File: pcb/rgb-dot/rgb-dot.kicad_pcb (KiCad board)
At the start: 2 copper layers, 7.6 x 8.9 mm, 4 parts, among them J1 HEADER-1x03, J2 HEADER-1x03, U1 WS2812B

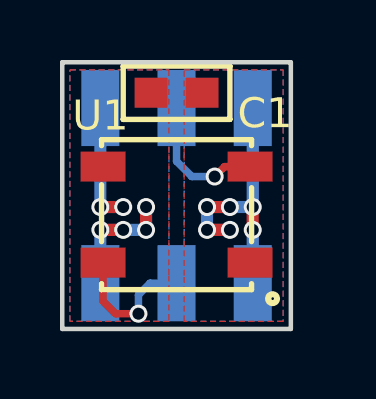
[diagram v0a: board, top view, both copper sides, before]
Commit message: Updated schematics
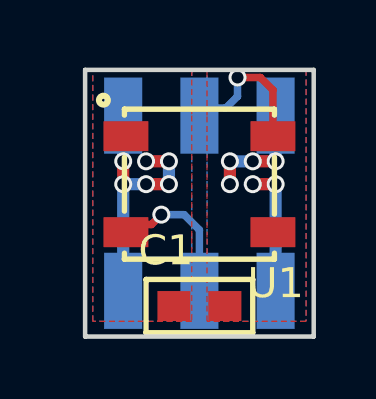
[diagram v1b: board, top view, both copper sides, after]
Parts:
- moved C1 7.15 mm to (149.4, 108.0), turned to 0 degrees
- moved J1 6.14 mm to (149.4, 107.4), turned to 180 degrees
- moved J2 5.64 mm to (149.4, 101.6), turned to 180 degrees
- moved U1 1.27 mm to (149.4, 103.9), turned to 180 degrees
